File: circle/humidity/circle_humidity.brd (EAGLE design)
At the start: 25.4 x 33 mm, 12 parts, among them IC1 ADA4075

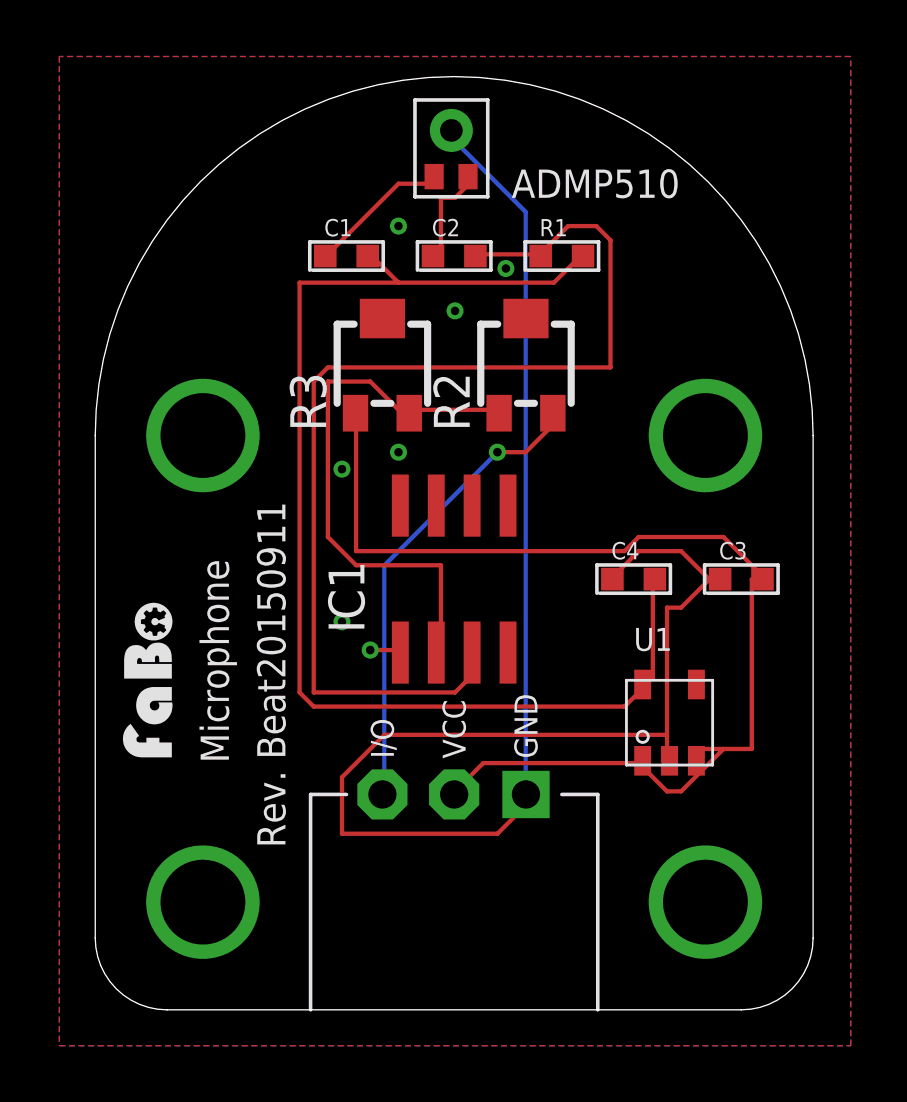
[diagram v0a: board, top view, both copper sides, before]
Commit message: Update circle
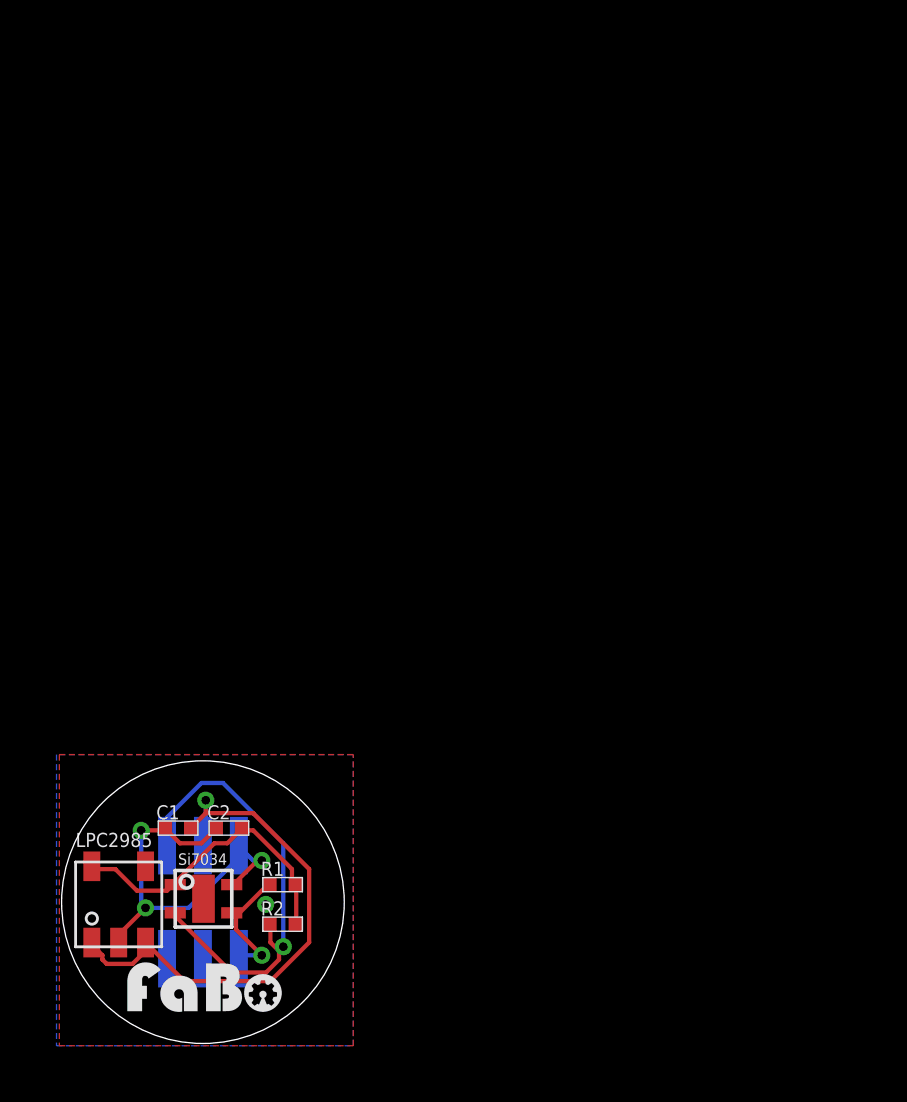
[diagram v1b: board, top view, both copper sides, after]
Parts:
- removed C3, C4: 1uf, GClue-Capacitor:0603
- removed IC1: ADA4075, analog-devices:SO8
- removed J1: (no value), FaBo-Template:FABO_BRICK_3PIN
- removed R3: (no value), rcl:RTRIM3202
- removed U$1: ANALOGDEVICES-ADMP510, FaBo-Mems:ANALOGDEVICES-ADMP510
- removed U1: (no value), FaBo-Supply:SOT_23_5
- added LPC2985: (no value), FaBo-Supply:TI-LP2985
- added U$5: FABO-NANO, FaBo-Template:FABO-NANO
- added U$6: SILICONLABS-SI7034, FaBo-Mems:SILICONLABS-SI7034
- C1: value 0.1uF -> 1uf; device FaBo-Capacitor:0603 -> FaBo-Capacitor:0402
- C2: value 1uf -> 2.2pf; device FaBo-Capacitor:0603 -> FaBo-Capacitor:0402
- R1: value 10k -> 4.7K; device FaBo-Resistors:0603 -> FaBo-Resistors:0402
- R2: value (none) -> 4.7K; device rcl:RTRIM3202 -> FaBo-Resistors:0402
- U$2: device FaBo:LOGO_FABO_S -> FaBo-etc:LOGO_FABO_S
- moved R1 24.3 mm to (7.90, 5.70)
- moved C2 21.8 mm to (6.00, 7.70)
- moved R2 21.6 mm to (7.90, 4.30)
- moved C1 21.1 mm to (4.20, 7.70)
- moved U$2 11.9 mm to (5.20, 1.20), turned to 0 degrees
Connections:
- removed net 3V3: C1.2, C4.2, R1.2, U1.5
- removed net 5V: C3.2, J1.VCC, R3.1, U1.1, U1.3
- removed net N$1: C2.1, U$1.2
- removed net N$2: C2.2, IC1.3, R1.1
- removed net N$3: IC1.1, J1.IN/OUT, R2.3
- removed net N$4: IC1.2, R2.1, R3.3
- removed net N$5: C1.1, U$1.1
- removed net V+: IC1.8
- removed net V-: IC1.4
- new net 1.8V: C2.P$2, LPC2985.5, R1.P$2, R2.P$2, U$6.1
- new net 3.3V: C1.P$2, LPC2985.1, LPC2985.3, U$5.VCC
- new net SCL: R2.P$1, U$5.0, U$6.2
- new net SDA: R1.P$1, U$5.1, U$6.4
- net GND: now also C1.P$1, C2.P$1, LPC2985.2, U$5.GND, U$6.5; no longer C3.1, C4.1, J1.GND, U$1.3, U1.2
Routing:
- net 3V3: track 43.6 -> 0.00 mm
- net GND: track 58.1 -> 14.6 mm, vias 6 -> 4
- net 5V: track 40.4 -> 0.00 mm
- net N$2: track 38.3 -> 0.00 mm
- net N$4: track 19.7 -> 0.00 mm
- net 3.3V: track 0.00 -> 19.6 mm, vias 0 -> 1
- net N$3: track 18.2 -> 0.00 mm, vias 2 -> 0
- net SCL: track 0.00 -> 16.6 mm, vias 0 -> 1
- net 1.8V: track 0.00 -> 11.0 mm
- net N$5: track 5.00 -> 0.00 mm
- net SDA: track 0.00 -> 4.49 mm, vias 0 -> 1
- net N$1: track 3.75 -> 0.00 mm
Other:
- board size 25.4 x 33 mm -> 10 x 10 mm
- board text removed: "ADMP510"
- board text removed: "Microphone"
- board text removed: "Rev. Beat20150911"
